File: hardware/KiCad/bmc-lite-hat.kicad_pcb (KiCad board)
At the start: 2 copper layers, 2 parts

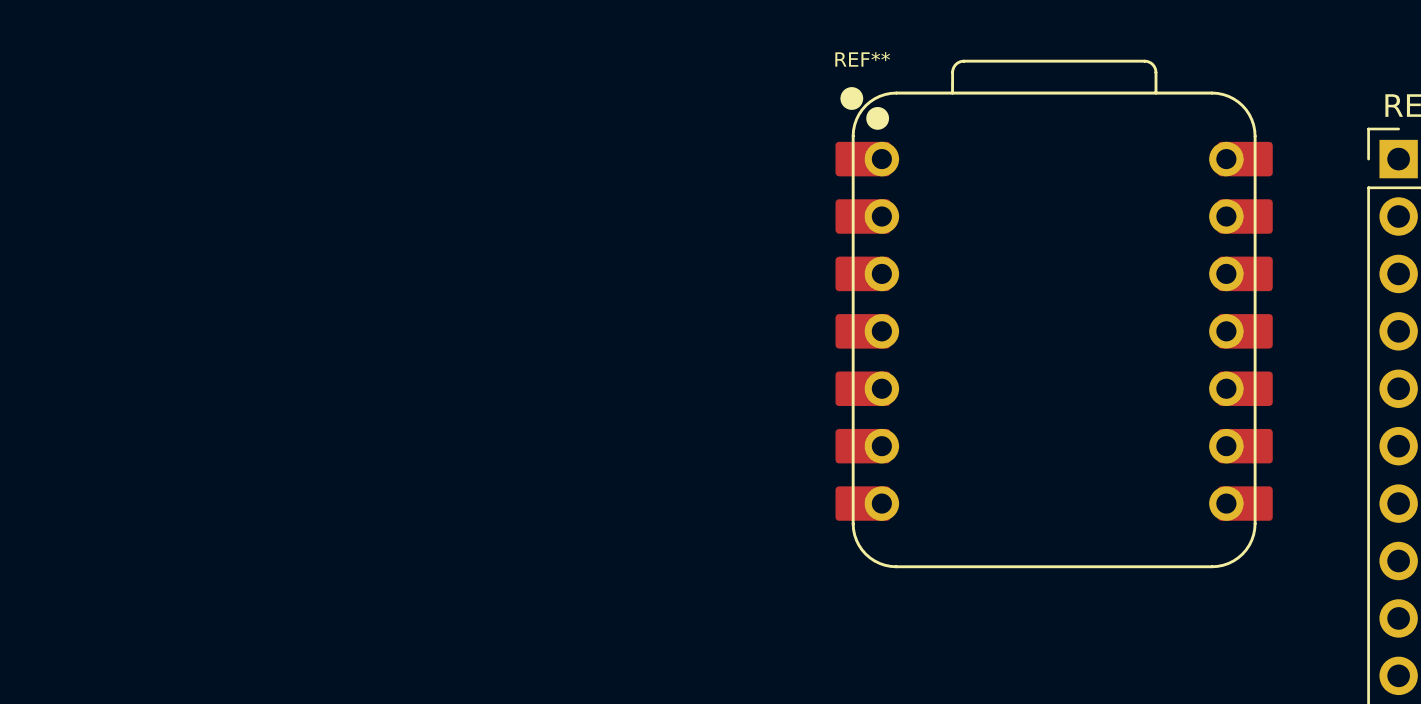
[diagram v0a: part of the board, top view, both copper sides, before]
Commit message: Update KiCad from Haruna
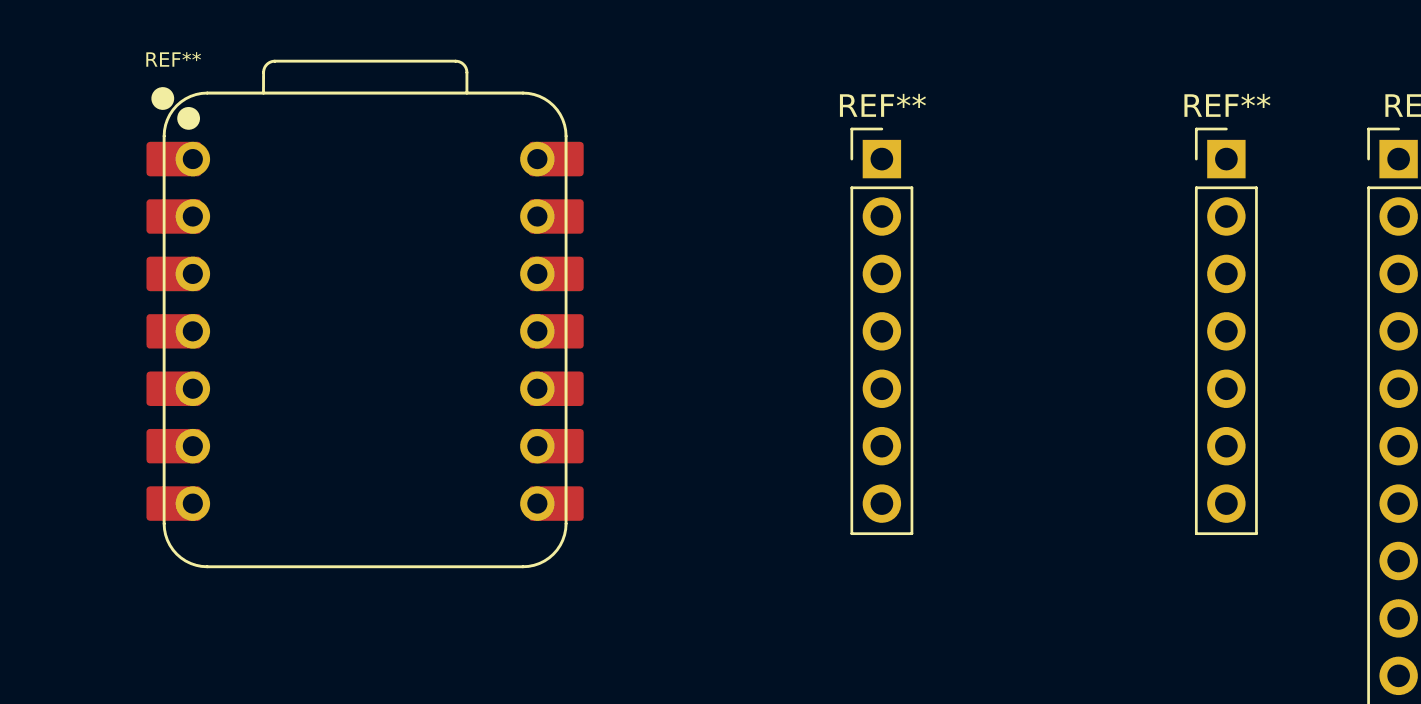
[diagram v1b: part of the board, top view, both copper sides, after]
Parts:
- added REF**: PinHeader_1x07_P2.54mm_Vertical, Connector_PinHeader_2.54mm:PinHeader_1x07_P2.54mm_Vertical, F.Cu at (185.4, 45.7)
- added REF**: PinHeader_1x07_P2.54mm_Vertical, Connector_PinHeader_2.54mm:PinHeader_1x07_P2.54mm_Vertical, F.Cu at (170.2, 45.7)
- moved REF** 30.5 mm to (147.3, 53.3)
